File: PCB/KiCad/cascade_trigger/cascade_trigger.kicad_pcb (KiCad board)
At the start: 2 copper layers, 144.8 x 77.5 mm, 69 parts, among them J1 Power_In, J2 Conn_02x07_Odd_Even, U2 Teensy3.6

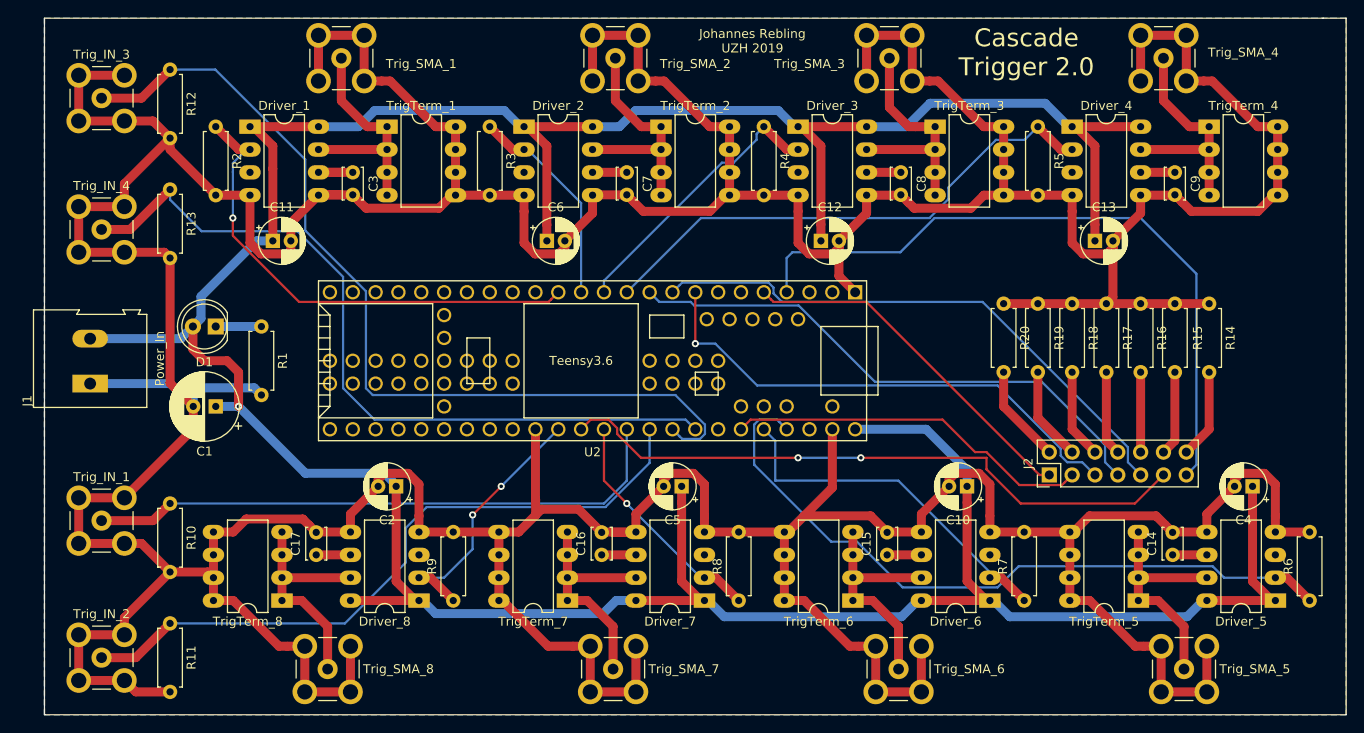
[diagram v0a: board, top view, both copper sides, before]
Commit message: 'quick' fix for OR microscope
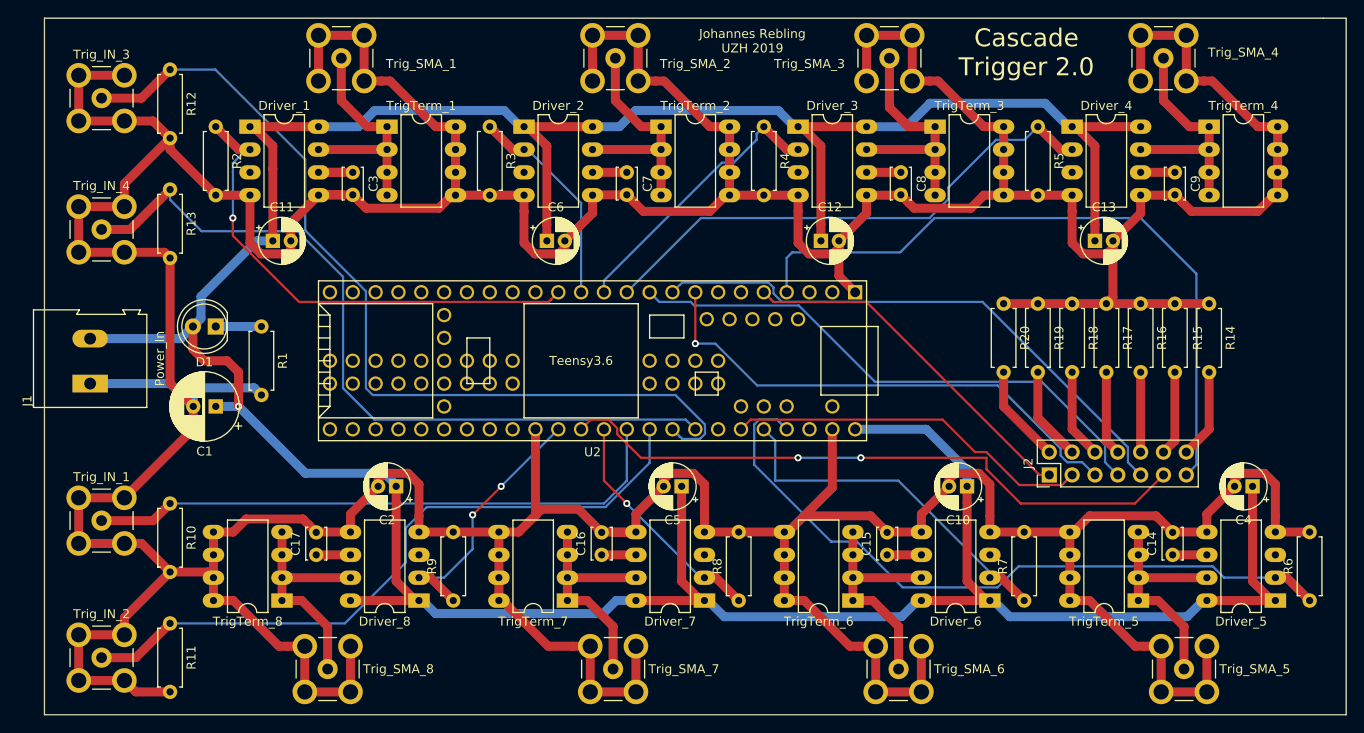
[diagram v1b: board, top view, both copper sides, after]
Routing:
- removed copper zone on B.Cu, net GND
- removed copper zone on F.Cu, net GND
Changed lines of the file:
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@@
   (segment (start 29.21 10.02137) (end 32.718629 13.529999) (width 0.25) (layer B.Cu) (net 116))
   (segment (start 29.21 8.89) (end 29.21 10.02137) (width 0.25) (layer B.Cu) (net 116))
-  (zone (net 2) (net_name GND) (layer F.Cu) (hatch edge 0.508)
-    (connect_pads (clearance 0.508))
-    (min_thickness 0.254)
-    (fill yes (arc_segments 32) (thermal_gap 0.508) (thermal_bridge_width 0.508))
-    (polygon
-      (pts
-        (xy 15.24 -10.16) (xy 160.02 -10.16) (xy 160.02 67.31) (xy 15.24 67.31)
-      )
-    )
-  )
-  (zone (net 2) (net_name GND) (layer B.Cu) (hatch edge 0.508)
-    (connect_pads (clearance 0.508))
-    (min_thickness 0.254)
-    (fill yes (arc_segments 32) (thermal_gap 0.508) (thermal_bridge_width 0.508))
-    (polygon
-      (pts
-        (xy 160.02 -10.16) (xy 15.24 -10.16) (xy 15.24 67.31) (xy 160.02 67.31)
-      )
-    )
-  )
 )
